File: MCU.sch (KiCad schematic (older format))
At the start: 29 parts, among them SW3 SW_Push, SW4 SW_Push, U10 ESP32-WROOM-32U, U6 STM32F730R8T6, U7 W25Q128JVSIQ, U9 FS35ND01G-S1Y2QWFI000, Y1 Q13FC1350000400, Y2 Crystal_GND24

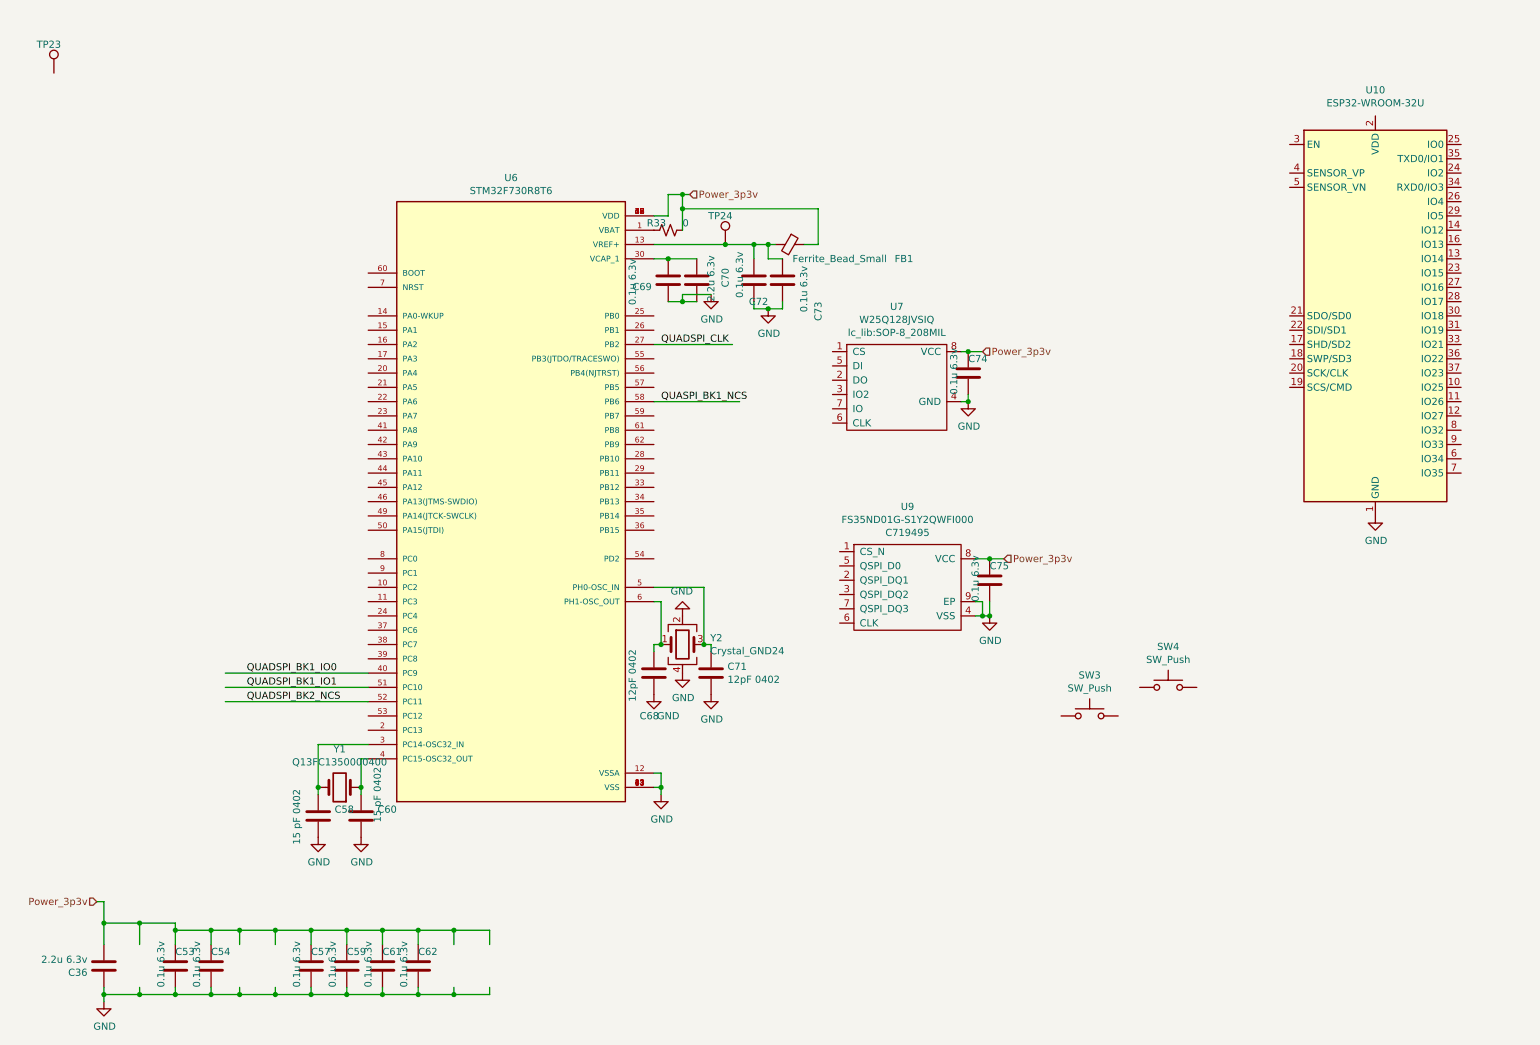
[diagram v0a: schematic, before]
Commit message: Much layout wow.
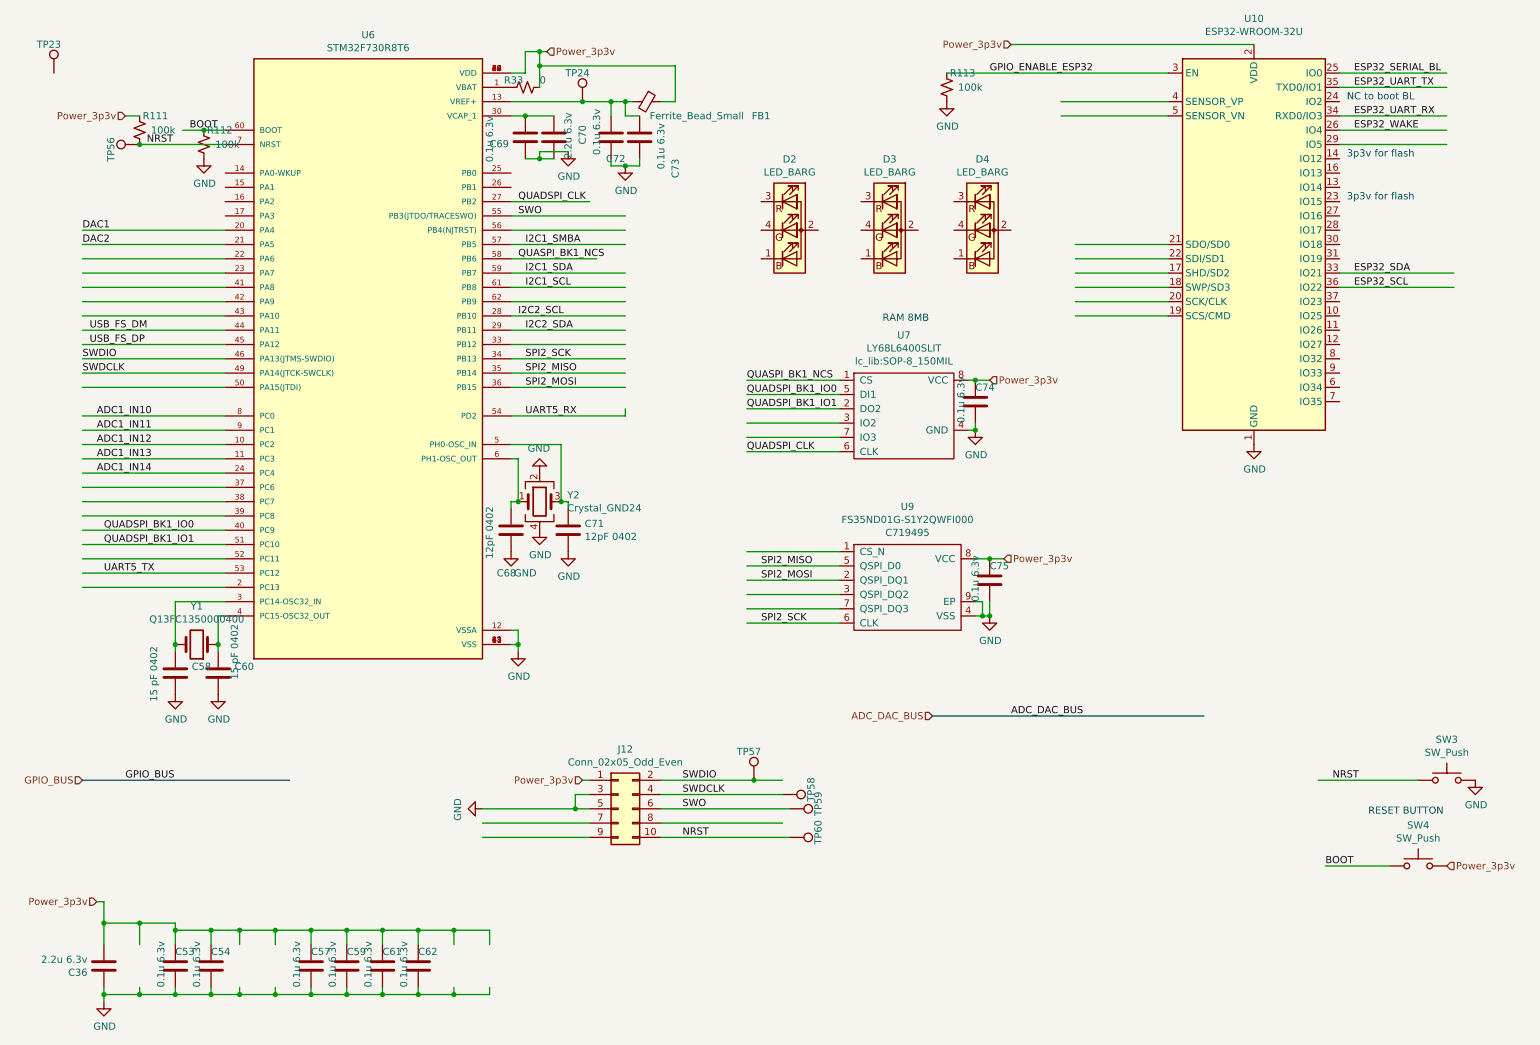
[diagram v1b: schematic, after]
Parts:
- removed U7: W25Q128JVSIQ, lc_lib:SOP-8_208MIL, symbol SmartBattery:W25Q128JVSIQ
- added D2, D3, D4: LED_BARG, LED_THT:LED_D5.0mm-4_RGB_Wide_Pins, symbol Device:LED_BARG
- added J12: Conn_02x05_Odd_Even, Connector_PinHeader_1.27mm:PinHeader_2x05_P1.27mm_Vertical_SMD, symbol Connector_Generic:Conn_02x05_Odd_Even
- added R111, R112, R113: 100k, lc_lib:0402_R, symbol Device:R_Small_US
- added TP56, TP57, TP58, TP59, TP60: TestPoint, TestPoint:TestPoint_Pad_D2.0mm, symbol Connector:TestPoint
- added U7: LY68L6400SLIT, lc_lib:SOP-8_150MIL, symbol SmartBattery:LY68L6400SLIT
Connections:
- net labels added: ADC1_IN10, ADC1_IN11, ADC1_IN12, ADC1_IN13, ADC1_IN14, ADC_DAC_BUS, BOOT, DAC1, DAC2, ESP32_SCL, ESP32_SDA, ESP32_SERIAL_BL, ESP32_UART_RX, ESP32_UART_TX, ESP32_WAKE, GPIO_BUS, GPIO_ENABLE_ESP32, I2C1_SCL, I2C1_SDA, I2C1_SMBA, I2C2_SCL, I2C2_SDA, NRST, SPI2_MISO, SPI2_MOSI, SPI2_SCK, SWDCLK, SWDIO, SWO, UART5_RX, UART5_TX, USB_FS_DM, USB_FS_DP
- net labels removed: QUADSPI_BK2_NCS
- wire segments 110 -> 194
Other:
- note added: "3p3v for flash"
- note added: "NC to boot BL"
- note added: "RAM 8MB\n"
- note added: "RESET BUTTON\n"
- moved on the sheet: C58, C60, C68, C69, C70, C71, C72, C73, C74, FB1, R33, SW3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
